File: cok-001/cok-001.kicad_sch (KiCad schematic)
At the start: 137 parts, among them J3209 ATA Power, J3221 ATA0 for BD, J3301 USB_A_Stacked, J3302 USB_A_Stacked, J3401 Conn_01x22_Pin, Q2401 DTC144E, Q2402 SI2303BDS, U2101 ADT7461A0002RMZR, U2105 TC7WP3125FK, U2108 ICS651MLFT, U2402 L7809, U2403 L7805, U2407 MM1593DFBEG, U3302 BU9869W, U6005 NCP511SN33T1G, U6006 NCP511SN18T1, U6009 NCP511SN33T1G, Y2101 24.576MHz

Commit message: ethernet
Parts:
- L3301, L3302, L3401, L3402: value L_Iron_Coupled_Small -> L_Iron_Coupled_Small_1243
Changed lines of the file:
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@@
 		(dnp no)
 		(property "Reference" "L3401"
-			(at 915.67 694.69 0)
+			(at 915.67 704.215 0)
 			(effects
 				(font
@@
 			)
 		)
-		(property "Value" "L_Iron_Coupled_Small"
-			(at 915.67 697.23 0)
+		(property "Value" "L_Iron_Coupled_Small_1243"
+			(at 915.67 697.865 0)
 			(effects
 				(font
@@
 			)
 		)
-		(property "Value" "L_Iron_Coupled_Small"
+		(property "Value" "L_Iron_Coupled_Small_1243"
 			(at 915.67 704.85 0)
 			(effects
@@
 		(dnp no)
 		(property "Reference" "L3301"
-			(at 236.22 67.31 0)
+			(at 236.22 57.785 0)
 			(effects
 				(font
@@
 			)
 		)
-		(property "Value" "L_Iron_Coupled_Small"
-			(at 236.22 64.77 0)
+		(property "Value" "L_Iron_Coupled_Small_1243"
+			(at 236.22 64.135 0)
 			(effects
 				(font
@@
 		(dnp no)
 		(property "Reference" "L3302"
-			(at 236.22 72.39 0)
+			(at 236.22 62.865 0)
 			(effects
 				(font
@@
 			)
 		)
-		(property "Value" "L_Iron_Coupled_Small"
-			(at 236.22 69.85 0)
+		(property "Value" "L_Iron_Coupled_Small_1243"
+			(at 236.22 69.215 0)
 			(effects
 				(font

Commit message: av
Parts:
- removed C2451: 470p 50V, Resistor_SMD:R_0402_1005Metric, symbol Device:C
- removed C2453, C2455: 220u 4V, Capacitor_SMD:CP_Elec_6.3x4.5, symbol Device:C_Polarized_US
- removed C2454, C2457, C2458: 1000u 4V, Capacitor_SMD:CP_Elec_8x6.9, symbol Device:C_Polarized_US
- removed C2456: 0.1u 16V, Capacitor_SMD:C_0603_1608Metric, symbol Device:C
- removed Q2401: DTC144E, Package_TO_SOT_SMD:SOT-323_SC-70, symbol Transistor_BJT:DTC144E
- removed Q2402: SI2303BDS, Package_TO_SOT_SMD:SOT-23, symbol Transistor_FET:TP0610T
- removed R2408: 150k, Resistor_SMD:R_0402_1005Metric, symbol Device:R_US
- removed R2447, R2448, R2449, R2450, R2451, R2452: 75, Resistor_SMD:R_0603_1608Metric, symbol Device:R_US
- removed U2402: L7809, Package_TO_SOT_SMD:TO-252-2, symbol Regulator_Linear:L7809
- removed U2403: L7805, Package_TO_SOT_SMD:TO-252-2, symbol Regulator_Linear:L7805
- removed U2406: ~, Package_QFP:TQFP-100_14x14mm_P0.5mm, symbol PS3:CXM4024
- removed U2407: MM1593DFBEG, Package_SO:SOP-8_3.9x4.9mm_P1.27mm, symbol PS3:MM159X
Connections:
- net HDMI_MCLK0 renamed HDMI_MCLKO0
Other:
- added sheet AV Out (av.kicad_sch)

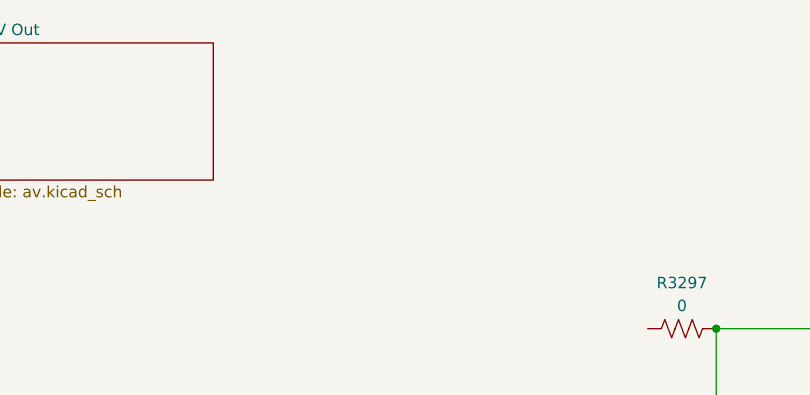
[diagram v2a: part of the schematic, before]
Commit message: row c and d
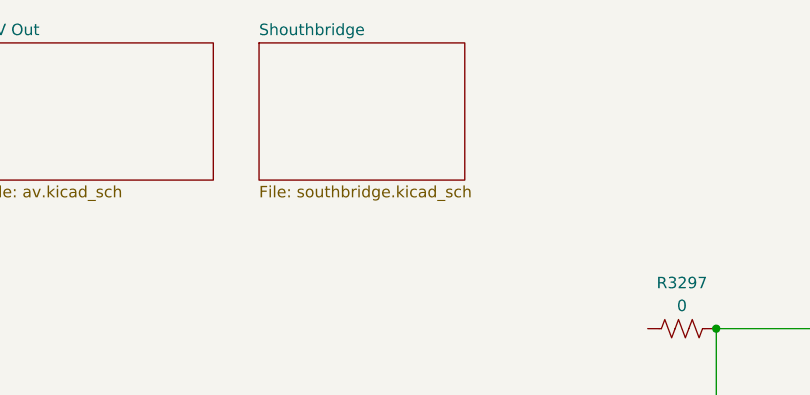
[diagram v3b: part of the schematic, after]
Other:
- added sheet Shouthbridge (southbridge.kicad_sch)
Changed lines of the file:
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@@
+	)
+	(sheet
+		(at 364.49 13.97)
+		(size 22.86 15.24)
+		(fields_autoplaced yes)
+		(stroke
+			(width 0.1524)
+			(type solid)
+		)
+		(fill
+			(color 0 0 0 0.0000)
+		)
+		(property "Sheetname" "Shouthbridge"
+			(at 364.49 13.2584 0)
+			(effects
+				(font
+					(size 1.27 1.27)
+				)
+				(justify left bottom)
+			)
+		)
+		(property "Sheetfile" "southbridge.kicad_sch"
+			(at 364.49 29.7946 0)
+			(effects
+				(font
+					(size 1.27 1.27)
+				)
+				(justify left top)
+			)
+		)
+		(instances
+			(project "cok-001"
+				(path "/976eb78d-8215-4cc0-9d72-f9d535c7970b"
+					(page "13")
+				)
+			)
+		)
 	)
 	(sheet
